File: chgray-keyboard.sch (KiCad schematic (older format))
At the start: 1 part, among them U1 Teensy2.0_(C)

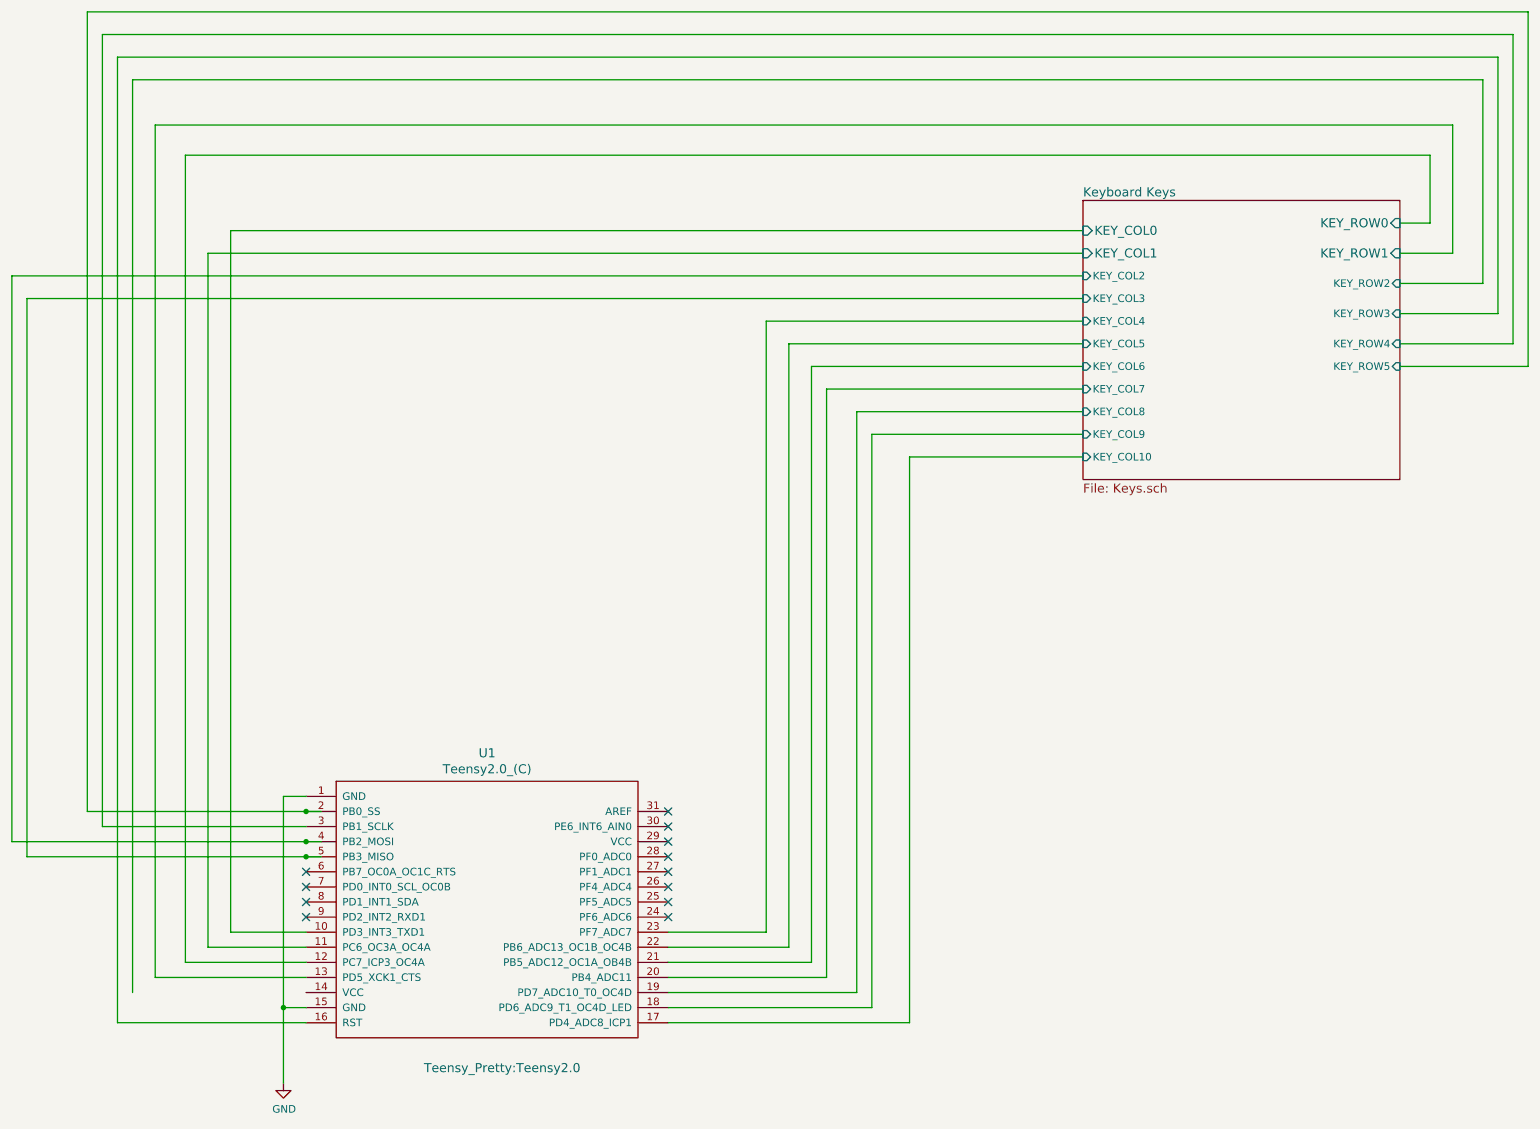
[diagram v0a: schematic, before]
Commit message: laying out the keys with logan
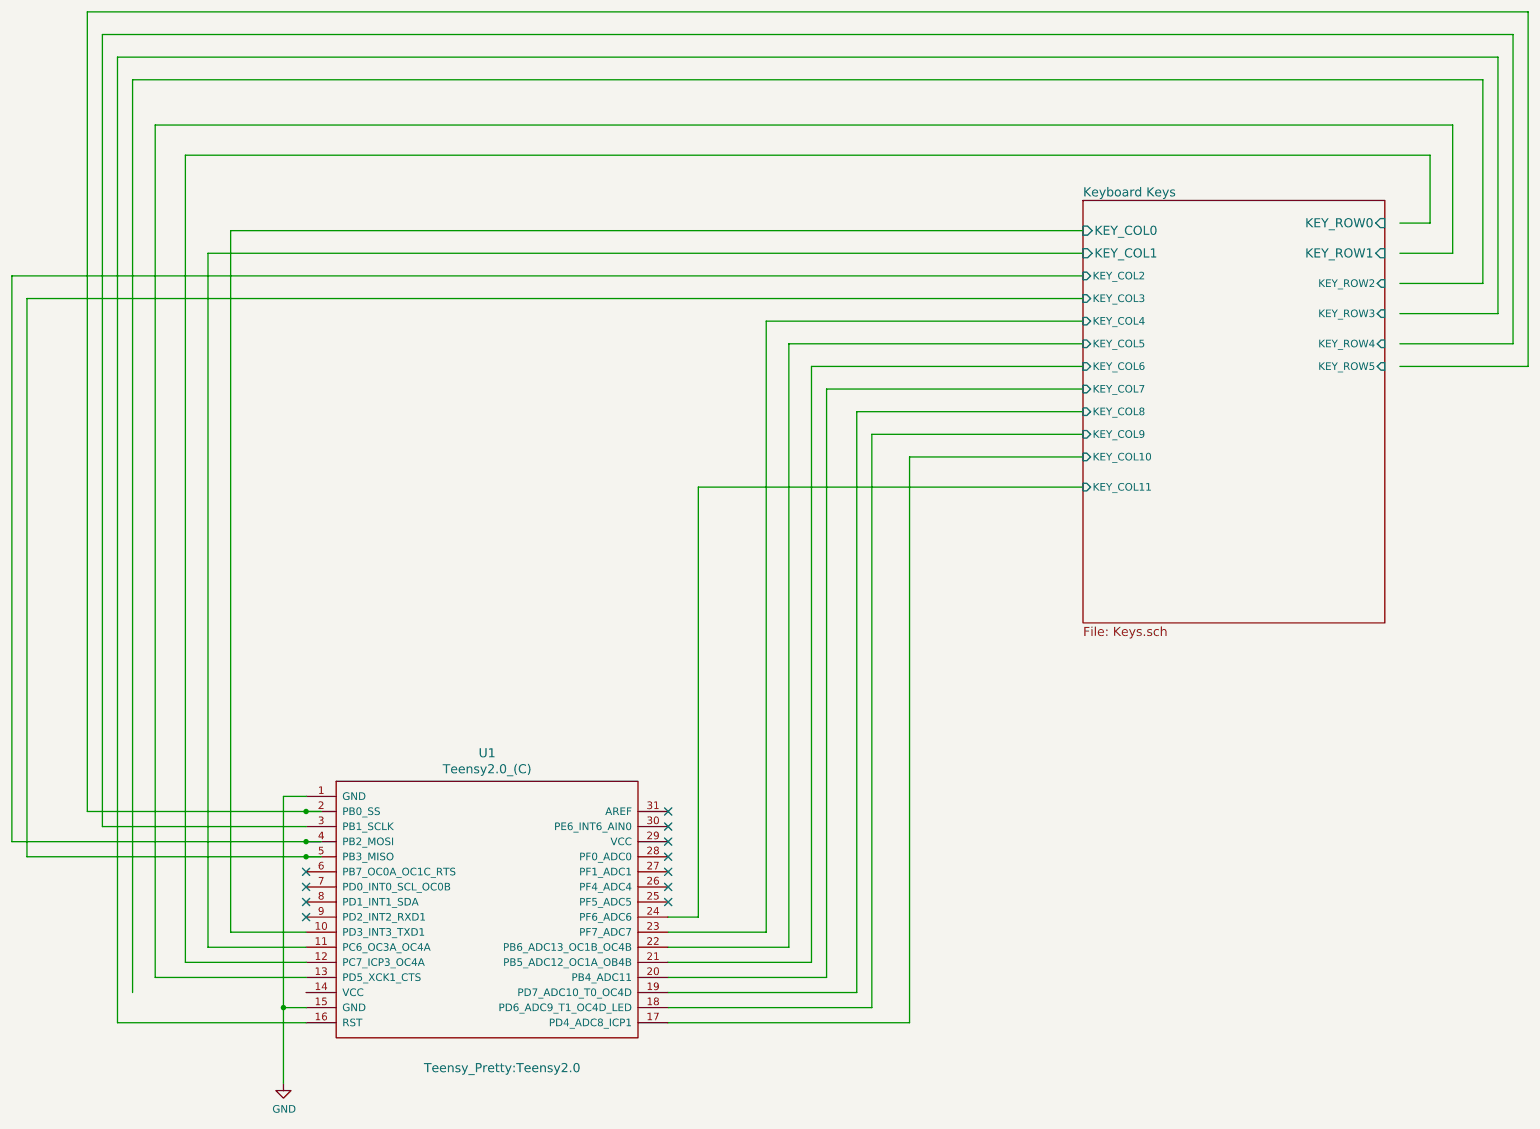
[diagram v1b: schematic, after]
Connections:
- wire segments 69 -> 72
- no-connect marks 12 -> 11
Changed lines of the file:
@@
 $EndDescr
 $Sheet
-S 7300 1800 2100 1850
+S 7300 1800 2000 2800
 U 589645BF
 F0 "Keyboard Keys" 60
 F1 "Keys.sch" 60
 F2 "KEY_COL0" I L 7300 2000 60
-F3 "KEY_ROW0" I R 9400 1950 60
-F4 "KEY_ROW1" I R 9400 2150 60
+F3 "KEY_ROW0" I R 9300 1950 60
+F4 "KEY_ROW1" I R 9300 2150 60
 F5 "KEY_COL1" I L 7300 2150 60
-F6 "KEY_ROW2" I R 9400 2350 50
-F7 "KEY_ROW3" I R 9400 2550 50
-F8 "KEY_ROW4" I R 9400 2750 50
-F9 "KEY_ROW5" I R 9400 2900 50
+F6 "KEY_ROW2" I R 9300 2350 50
+F7 "KEY_ROW3" I R 9300 2550 50
+F8 "KEY_ROW4" I R 9300 2750 50
+F9 "KEY_ROW5" I R 9300 2900 50
 F10 "KEY_COL2" I L 7300 2300 50
 F11 "KEY_COL3" I L 7300 2450 50
@@
 F17 "KEY_COL9" I L 7300 3350 50
 F18 "KEY_COL10" I L 7300 3500 50
+F19 "KEY_COL11" I L 7300 3700 50
 $EndSheet
 Wire Wire Line
@@
 NoConn ~ 4550 6350
 NoConn ~ 4550 6450
-NoConn ~ 4550 6550
 NoConn ~ 2150 6250
 NoConn ~ 2150 6350
@@
 	2000 7150 2000 7650
 Connection ~ 2000 7150
+Wire Wire Line
+	7300 3700 4750 3700
+Wire Wire Line
+	4750 3700 4750 6550
+Wire Wire Line
+	4750 6550 4550 6550
 $EndSCHEMATC
